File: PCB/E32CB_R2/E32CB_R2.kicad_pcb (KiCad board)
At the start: 2 copper layers, 111.3 x 90.9 mm, 91 parts, among them J1 GPIO_HEADER, J10 S, J11 Q4, J12 S, J13 Q3, J14 S, J15 Q8, J16 S, J17 Q7, J18 S, J19 Q6, J2 Power, J20 S, J21 Q5, J22 S, J3 USB_B, J4 USB +5V, J5 NEXTION, J6 I2C, J7 Q1, J8 S, J9 Q2, Q1 S8050, Q10 IRLR2905, Q2 S8050, Q3 IRLR2905, Q4 IRLR2905, Q5 IRLR2905, Q6 IRLR2905, Q7 IRLR2905, Q8 IRLR2905, Q9 IRLR2905, U1 ESP32-WROOM-32, X1 12MHz

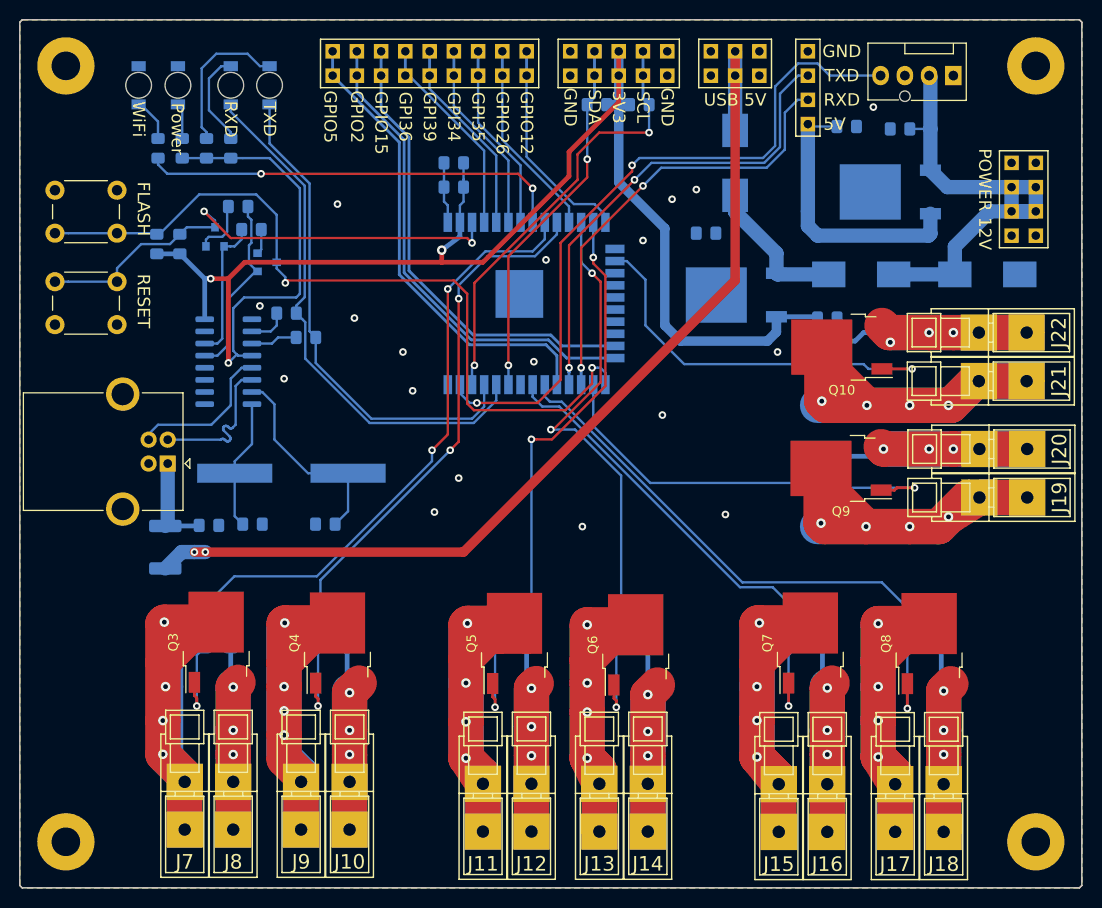
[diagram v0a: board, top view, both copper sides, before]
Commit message: track update
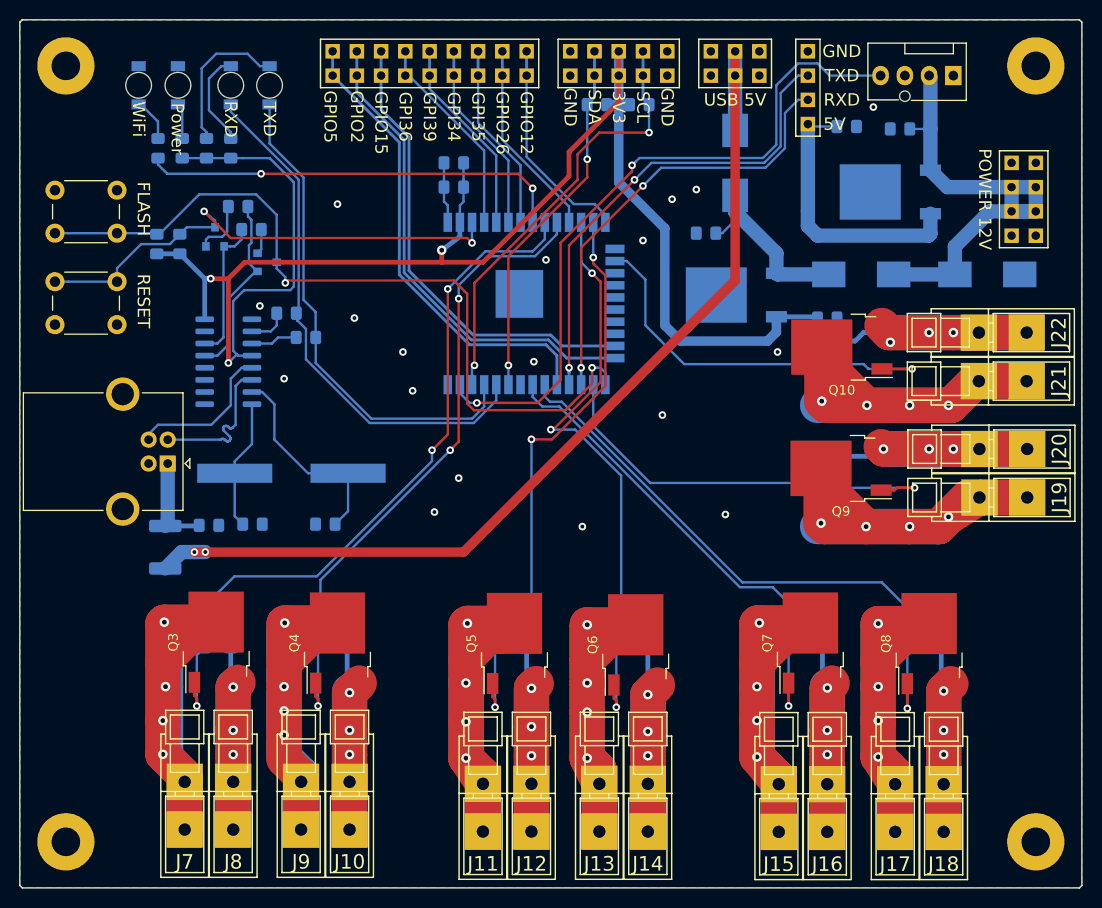
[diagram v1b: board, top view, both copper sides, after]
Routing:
- net Net-(3V3stabilizer1-Pad1): track 15.5 -> 18.9 mm
- net +3V3: track 181.2 -> 180.3 mm
- net /RXD: track 56.0 -> 55.5 mm
- removed copper zone on B.Cu, net GND

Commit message: refill zones
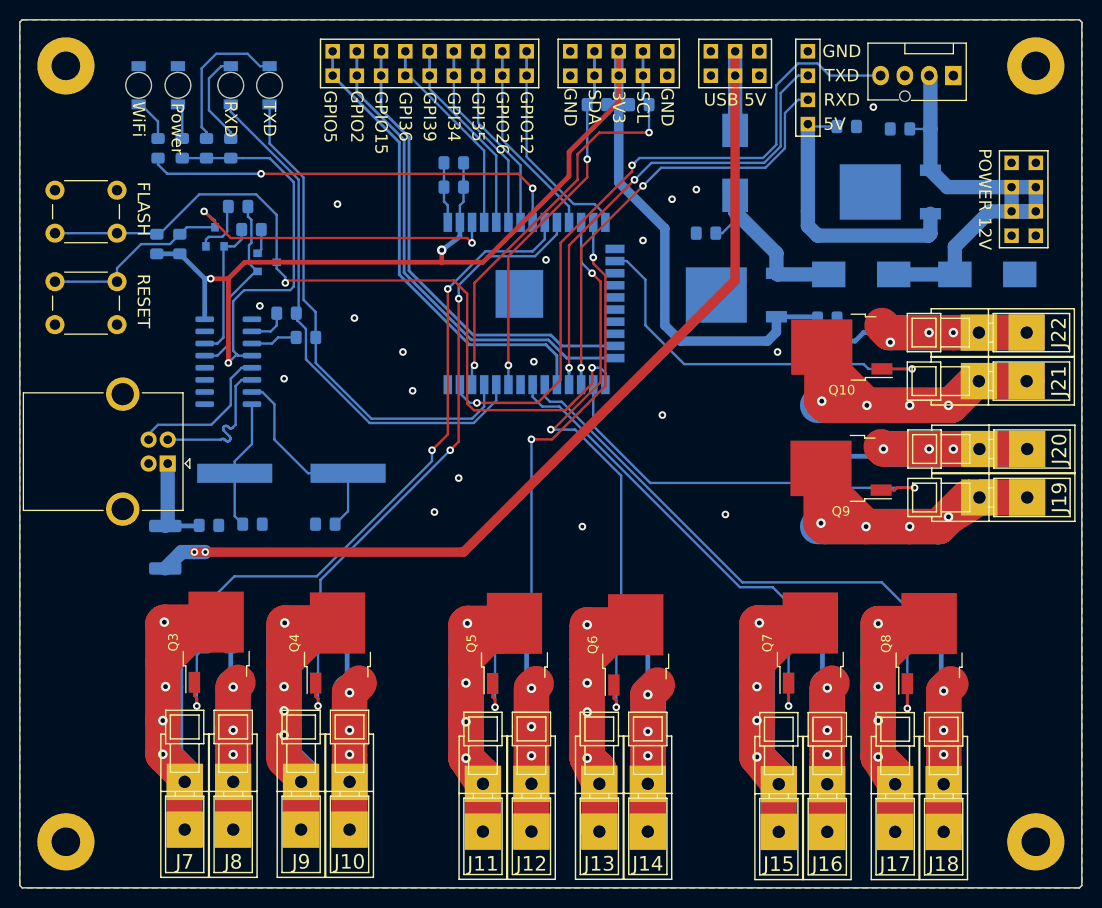
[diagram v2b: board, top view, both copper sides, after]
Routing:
- added copper zone on B.Cu, net GND
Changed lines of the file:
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@@
   )
   (setup
-    (last_trace_width 0.3)
+    (last_trace_width 1)
     (user_trace_width 0.3)
     (user_trace_width 0.5)
@@
     (user_trace_width 3.7)
     (trace_clearance 0.2)
-    (zone_clearance 0.508)
+    (zone_clearance 0.3)
     (zone_45_only no)
     (trace_min 0.1)
@@
   (segment (start 112.014 98.994) (end 115.5 98.994) (width 0.5) (layer B.Cu) (net 84))
   (zone (net 8) (net_name GND) (layer F.Cu) (hatch edge 0.508)
-    (connect_pads (clearance 0.508))
+    (connect_pads (clearance 0.3))
+    (min_thickness 0.25)
+    (fill yes (arc_segments 16) (thermal_gap 0.508) (thermal_bridge_width 0.508))
+    (polygon
+      (pts
+        (xy 96.774 136.652) (xy 96.774 46.228) (xy 97.028 45.974) (xy 207.772 45.974) (xy 208.026 46.228)
+        (xy 208.026 136.652) (xy 207.772 136.906) (xy 97.028 136.906)
+      )
+    )
+  )
+  (zone (net 8) (net_name GND) (layer B.Cu) (hatch edge 0.508)
+    (connect_pads (clearance 0.3))
     (min_thickness 0.25)
     (fill yes (arc_segments 16) (thermal_gap 0.508) (thermal_bridge_width 0.508))
